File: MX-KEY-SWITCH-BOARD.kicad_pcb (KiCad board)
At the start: 2 copper layers, 97 x 101.2 mm, 112 parts, among them J1 Conn_01x06, J10 Conn_01x06, J11 Conn_01x06, J12 Conn_01x06, J13 Conn_01x06, J14 Conn_01x06, J15 Conn_01x06, J16 Conn_01x06, J17 Conn_01x06, J18 Conn_01x06, J19 Conn_01x06, J2 Conn_01x06, J20 Conn_01x06, J21 Conn_01x06, J22 Conn_01x06, J23 Conn_01x06, J24 Conn_01x06, J25 Conn_01x06, J26 Conn_01x06, J27 Conn_01x06, J28 Conn_01x06, J29 Conn_01x06, J3 Conn_01x06, J30 Conn_01x06, J31 Conn_01x06, J32 Conn_01x06, J33 Conn_01x06, J34 Conn_01x06, J35 Conn_01x06, J36 Conn_01x06, J37 Conn_01x06, J38 Conn_01x06, J39 Conn_01x06, J4 Conn_01x06, J40 Conn_01x06, J41 Conn_01x06, J42 Conn_01x06, J43 Conn_01x06, J44 Conn_01x06, J45 Conn_01x06, J46 Conn_01x06, J47 Conn_01x06, J48 Conn_01x06, J49 Conn_01x06, J5 Conn_01x06, J50 Conn_01x06, J51 Conn_01x06, J52 Conn_01x06, J53 Conn_01x06, J54 Conn_01x06, J55 Conn_01x06, J56 Conn_01x06, J57 Conn_01x06, J58 Conn_01x06, J59 Conn_01x06, J6 Conn_01x06, J60 Conn_01x06, J61 Conn_01x06, J62 Conn_01x06, J63 Conn_01x06, J64 Conn_01x06, J7 Conn_01x06, J8 Conn_01x06, J9 Conn_01x06, SW1 SW_Push, SW10 SW_Push, SW11 SW_Push, SW12 SW_Push, SW13 SW_Push, SW14 SW_Push, SW15 SW_Push, SW16 SW_Push, SW2 SW_Push, SW3 SW_Push, SW4 SW_Push, SW5 SW_Push, SW6 SW_Push, SW7 SW_Push, SW8 SW_Push, SW9 SW_Push

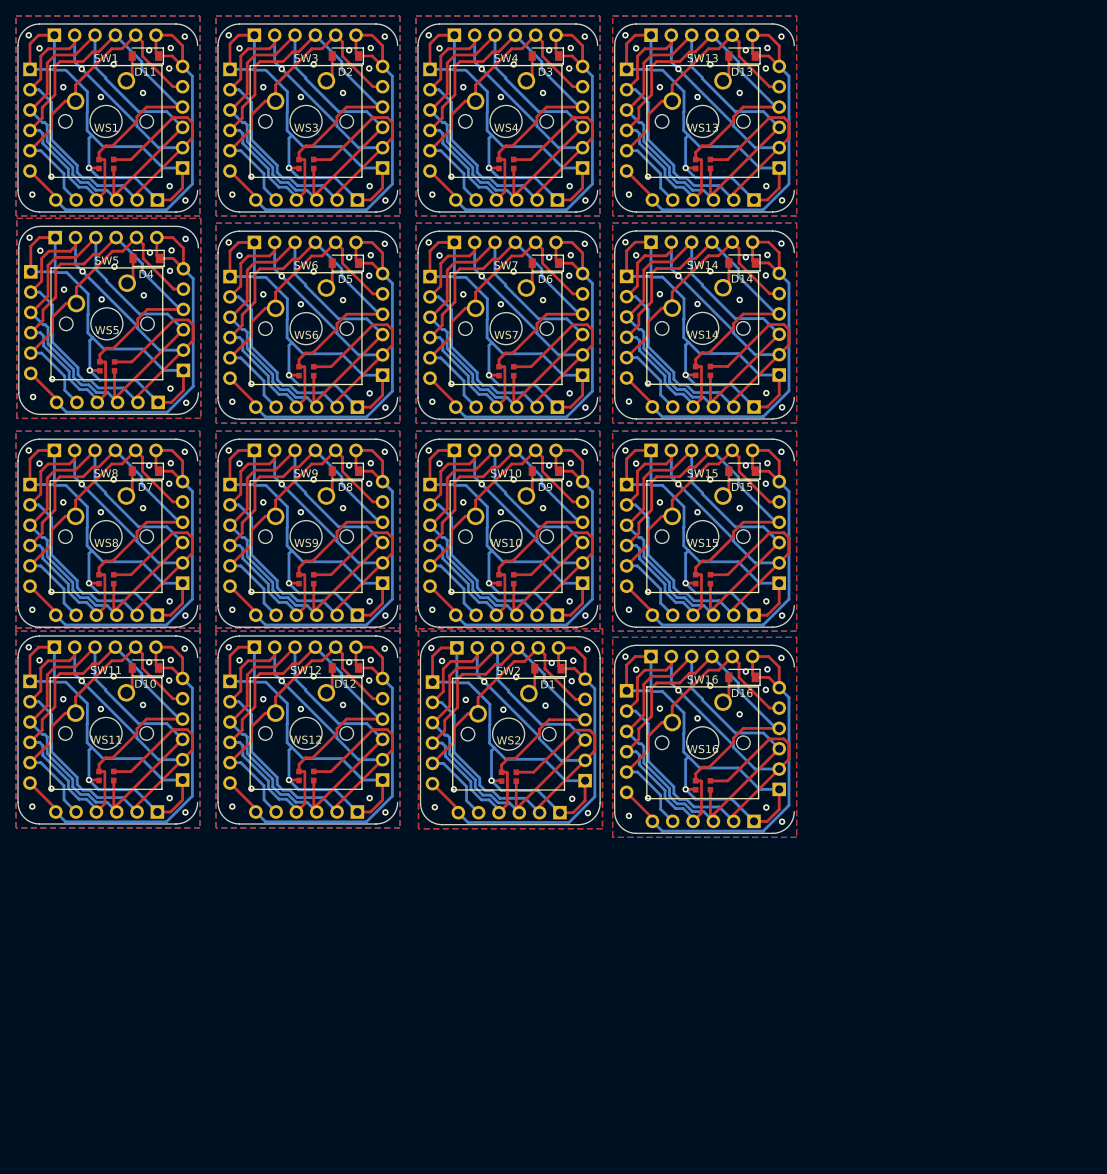
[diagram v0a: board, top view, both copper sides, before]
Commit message: fix
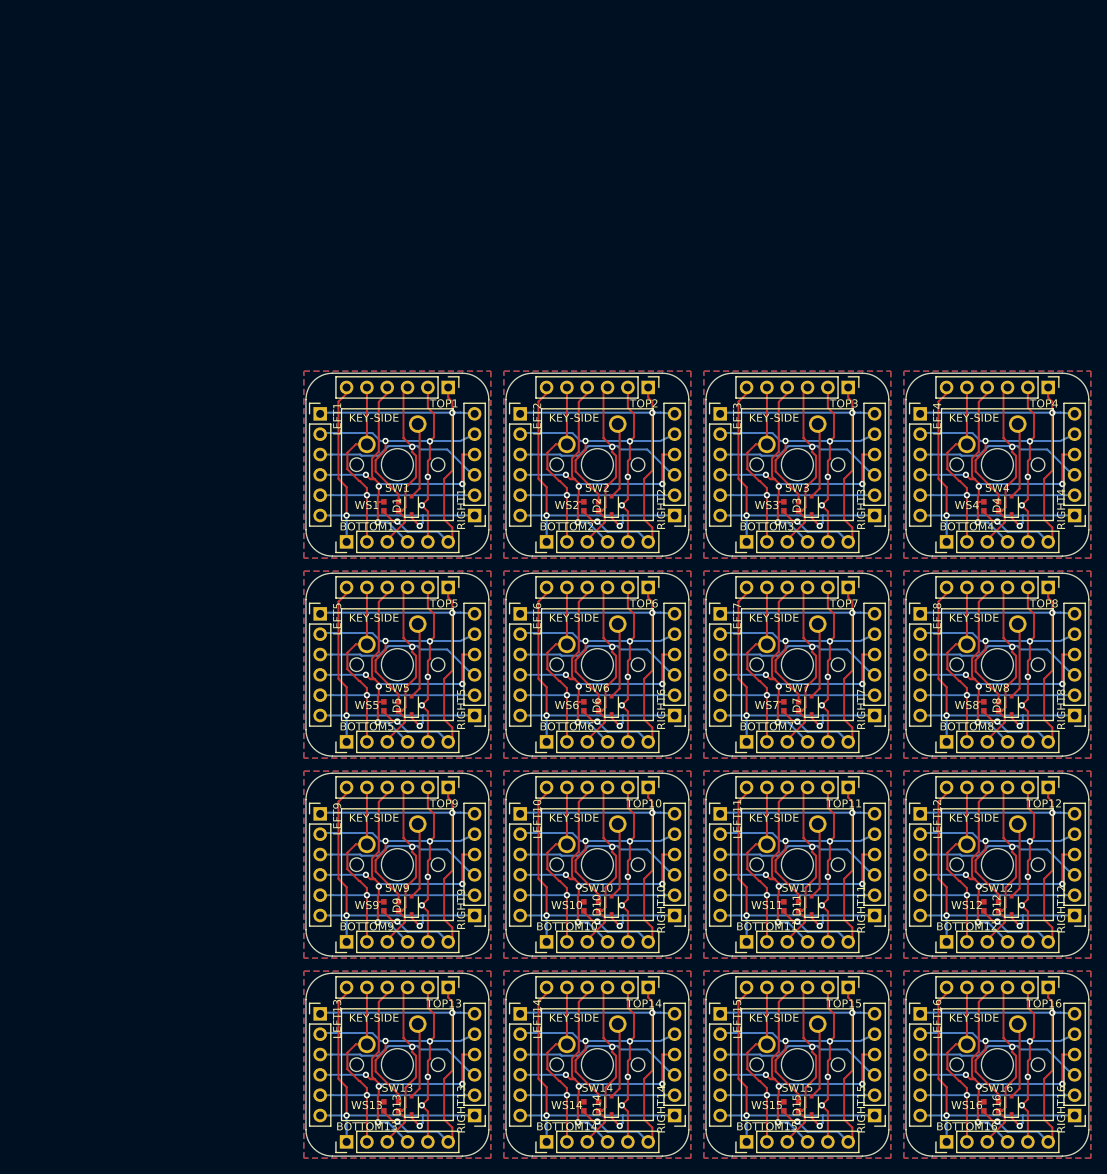
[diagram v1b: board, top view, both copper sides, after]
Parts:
- removed J1, J10, J11, J12, J13, J14, J15, J16, J17, J18, J19, J2, J20, J21, J22, J23, J24, J25, J26, J27, J28, J29, J3, J30, J31, J32, J33, J34, J35, J36, J37, J38, J39, J4, J40, J41, J42, J43, J44, J45, J46, J47, J48, J49, J5, J50, J51, J52, J53, J54, J55, J56, J57, J58, J59, J6, J60, J61, J62, J63, J64, J7, J8, J9: Conn_01x06, Connector_PinHeader_2.54mm:PinHeader_1x06_P2.54mm_Vertical
- added BOTTOM1: Conn_01x06, Connector_PinHeader_2.54mm:PinHeader_1x06_P2.54mm_Vertical, F.Cu at (-8.89, 14.7)
- added BOTTOM10: Conn_01x06, Connector_PinHeader_2.54mm:PinHeader_1x06_P2.54mm_Vertical, F.Cu at (16.1, 64.7)
- added BOTTOM11: Conn_01x06, Connector_PinHeader_2.54mm:PinHeader_1x06_P2.54mm_Vertical, F.Cu at (41.1, 64.7)
- added BOTTOM12: Conn_01x06, Connector_PinHeader_2.54mm:PinHeader_1x06_P2.54mm_Vertical, F.Cu at (66.1, 64.7)
- added BOTTOM13: Conn_01x06, Connector_PinHeader_2.54mm:PinHeader_1x06_P2.54mm_Vertical, F.Cu at (-8.89, 89.7)
- added BOTTOM14: Conn_01x06, Connector_PinHeader_2.54mm:PinHeader_1x06_P2.54mm_Vertical, F.Cu at (16.1, 89.7)
- added BOTTOM15: Conn_01x06, Connector_PinHeader_2.54mm:PinHeader_1x06_P2.54mm_Vertical, F.Cu at (41.1, 89.7)
- added BOTTOM16: Conn_01x06, Connector_PinHeader_2.54mm:PinHeader_1x06_P2.54mm_Vertical, F.Cu at (66.1, 89.7)
- added BOTTOM2: Conn_01x06, Connector_PinHeader_2.54mm:PinHeader_1x06_P2.54mm_Vertical, F.Cu at (16.1, 14.7)
- added BOTTOM3: Conn_01x06, Connector_PinHeader_2.54mm:PinHeader_1x06_P2.54mm_Vertical, F.Cu at (41.1, 14.7)
- added BOTTOM4: Conn_01x06, Connector_PinHeader_2.54mm:PinHeader_1x06_P2.54mm_Vertical, F.Cu at (66.1, 14.7)
- added BOTTOM5: Conn_01x06, Connector_PinHeader_2.54mm:PinHeader_1x06_P2.54mm_Vertical, F.Cu at (-8.89, 39.7)
- added BOTTOM6: Conn_01x06, Connector_PinHeader_2.54mm:PinHeader_1x06_P2.54mm_Vertical, F.Cu at (16.1, 39.7)
- added BOTTOM7: Conn_01x06, Connector_PinHeader_2.54mm:PinHeader_1x06_P2.54mm_Vertical, F.Cu at (41.1, 39.7)
- added BOTTOM8: Conn_01x06, Connector_PinHeader_2.54mm:PinHeader_1x06_P2.54mm_Vertical, F.Cu at (66.1, 39.7)
- added BOTTOM9: Conn_01x06, Connector_PinHeader_2.54mm:PinHeader_1x06_P2.54mm_Vertical, F.Cu at (-8.89, 64.7)
- added LEFT1: Conn_01x06, Connector_PinHeader_2.54mm:PinHeader_1x06_P2.54mm_Vertical, F.Cu at (-12.2, -1.27)
- added LEFT10: Conn_01x06, Connector_PinHeader_2.54mm:PinHeader_1x06_P2.54mm_Vertical, F.Cu at (12.8, 48.7)
- added LEFT11: Conn_01x06, Connector_PinHeader_2.54mm:PinHeader_1x06_P2.54mm_Vertical, F.Cu at (37.8, 48.7)
- added LEFT12: Conn_01x06, Connector_PinHeader_2.54mm:PinHeader_1x06_P2.54mm_Vertical, F.Cu at (62.8, 48.7)
- added LEFT13: Conn_01x06, Connector_PinHeader_2.54mm:PinHeader_1x06_P2.54mm_Vertical, F.Cu at (-12.2, 73.7)
- added LEFT14: Conn_01x06, Connector_PinHeader_2.54mm:PinHeader_1x06_P2.54mm_Vertical, F.Cu at (12.8, 73.7)
- added LEFT15: Conn_01x06, Connector_PinHeader_2.54mm:PinHeader_1x06_P2.54mm_Vertical, F.Cu at (37.8, 73.7)
- added LEFT16: Conn_01x06, Connector_PinHeader_2.54mm:PinHeader_1x06_P2.54mm_Vertical, F.Cu at (62.8, 73.7)
- added LEFT2: Conn_01x06, Connector_PinHeader_2.54mm:PinHeader_1x06_P2.54mm_Vertical, F.Cu at (12.8, -1.27)
- added LEFT3: Conn_01x06, Connector_PinHeader_2.54mm:PinHeader_1x06_P2.54mm_Vertical, F.Cu at (37.8, -1.27)
- added LEFT4: Conn_01x06, Connector_PinHeader_2.54mm:PinHeader_1x06_P2.54mm_Vertical, F.Cu at (62.8, -1.27)
- added LEFT5: Conn_01x06, Connector_PinHeader_2.54mm:PinHeader_1x06_P2.54mm_Vertical, F.Cu at (-12.2, 23.7)
- added LEFT6: Conn_01x06, Connector_PinHeader_2.54mm:PinHeader_1x06_P2.54mm_Vertical, F.Cu at (12.8, 23.7)
- added LEFT7: Conn_01x06, Connector_PinHeader_2.54mm:PinHeader_1x06_P2.54mm_Vertical, F.Cu at (37.8, 23.7)
- added LEFT8: Conn_01x06, Connector_PinHeader_2.54mm:PinHeader_1x06_P2.54mm_Vertical, F.Cu at (62.8, 23.7)
- added LEFT9: Conn_01x06, Connector_PinHeader_2.54mm:PinHeader_1x06_P2.54mm_Vertical, F.Cu at (-12.2, 48.7)
- added RIGHT1: Conn_01x06, Connector_PinHeader_2.54mm:PinHeader_1x06_P2.54mm_Vertical, F.Cu at (7.11, 11.4)
- added RIGHT10: Conn_01x06, Connector_PinHeader_2.54mm:PinHeader_1x06_P2.54mm_Vertical, F.Cu at (32.1, 61.4)
- added RIGHT11: Conn_01x06, Connector_PinHeader_2.54mm:PinHeader_1x06_P2.54mm_Vertical, F.Cu at (57.1, 61.4)
- added RIGHT12: Conn_01x06, Connector_PinHeader_2.54mm:PinHeader_1x06_P2.54mm_Vertical, F.Cu at (82.1, 61.4)
- added RIGHT13: Conn_01x06, Connector_PinHeader_2.54mm:PinHeader_1x06_P2.54mm_Vertical, F.Cu at (7.11, 86.4)
- added RIGHT14: Conn_01x06, Connector_PinHeader_2.54mm:PinHeader_1x06_P2.54mm_Vertical, F.Cu at (32.1, 86.4)
- added RIGHT15: Conn_01x06, Connector_PinHeader_2.54mm:PinHeader_1x06_P2.54mm_Vertical, F.Cu at (57.1, 86.4)
- added RIGHT16: Conn_01x06, Connector_PinHeader_2.54mm:PinHeader_1x06_P2.54mm_Vertical, F.Cu at (82.1, 86.4)
- added RIGHT2: Conn_01x06, Connector_PinHeader_2.54mm:PinHeader_1x06_P2.54mm_Vertical, F.Cu at (32.1, 11.4)
- added RIGHT3: Conn_01x06, Connector_PinHeader_2.54mm:PinHeader_1x06_P2.54mm_Vertical, F.Cu at (57.1, 11.4)
- added RIGHT4: Conn_01x06, Connector_PinHeader_2.54mm:PinHeader_1x06_P2.54mm_Vertical, F.Cu at (82.1, 11.4)
- added RIGHT5: Conn_01x06, Connector_PinHeader_2.54mm:PinHeader_1x06_P2.54mm_Vertical, F.Cu at (7.11, 36.4)
- added RIGHT6: Conn_01x06, Connector_PinHeader_2.54mm:PinHeader_1x06_P2.54mm_Vertical, F.Cu at (32.1, 36.4)
- added RIGHT7: Conn_01x06, Connector_PinHeader_2.54mm:PinHeader_1x06_P2.54mm_Vertical, F.Cu at (57.1, 36.4)
- added RIGHT8: Conn_01x06, Connector_PinHeader_2.54mm:PinHeader_1x06_P2.54mm_Vertical, F.Cu at (82.1, 36.4)
- added RIGHT9: Conn_01x06, Connector_PinHeader_2.54mm:PinHeader_1x06_P2.54mm_Vertical, F.Cu at (7.11, 61.4)
- added TOP1: Conn_01x06, Connector_PinHeader_2.54mm:PinHeader_1x06_P2.54mm_Vertical, F.Cu at (3.81, -4.57)
- added TOP10: Conn_01x06, Connector_PinHeader_2.54mm:PinHeader_1x06_P2.54mm_Vertical, F.Cu at (28.8, 45.4)
- added TOP11: Conn_01x06, Connector_PinHeader_2.54mm:PinHeader_1x06_P2.54mm_Vertical, F.Cu at (53.8, 45.4)
- added TOP12: Conn_01x06, Connector_PinHeader_2.54mm:PinHeader_1x06_P2.54mm_Vertical, F.Cu at (78.8, 45.4)
- added TOP13: Conn_01x06, Connector_PinHeader_2.54mm:PinHeader_1x06_P2.54mm_Vertical, F.Cu at (3.81, 70.4)
- added TOP14: Conn_01x06, Connector_PinHeader_2.54mm:PinHeader_1x06_P2.54mm_Vertical, F.Cu at (28.8, 70.4)
- added TOP15: Conn_01x06, Connector_PinHeader_2.54mm:PinHeader_1x06_P2.54mm_Vertical, F.Cu at (53.8, 70.4)
- added TOP16: Conn_01x06, Connector_PinHeader_2.54mm:PinHeader_1x06_P2.54mm_Vertical, F.Cu at (78.8, 70.4)
- added TOP2: Conn_01x06, Connector_PinHeader_2.54mm:PinHeader_1x06_P2.54mm_Vertical, F.Cu at (28.8, -4.57)
- added TOP3: Conn_01x06, Connector_PinHeader_2.54mm:PinHeader_1x06_P2.54mm_Vertical, F.Cu at (53.8, -4.57)
- added TOP4: Conn_01x06, Connector_PinHeader_2.54mm:PinHeader_1x06_P2.54mm_Vertical, F.Cu at (78.8, -4.57)
- added TOP5: Conn_01x06, Connector_PinHeader_2.54mm:PinHeader_1x06_P2.54mm_Vertical, F.Cu at (3.81, 20.4)
- added TOP6: Conn_01x06, Connector_PinHeader_2.54mm:PinHeader_1x06_P2.54mm_Vertical, F.Cu at (28.8, 20.4)
- added TOP7: Conn_01x06, Connector_PinHeader_2.54mm:PinHeader_1x06_P2.54mm_Vertical, F.Cu at (53.8, 20.4)
- added TOP8: Conn_01x06, Connector_PinHeader_2.54mm:PinHeader_1x06_P2.54mm_Vertical, F.Cu at (78.8, 20.4)
- added TOP9: Conn_01x06, Connector_PinHeader_2.54mm:PinHeader_1x06_P2.54mm_Vertical, F.Cu at (3.81, 45.4)
- D1, D10, D11, D12, D13, D14, D15, D16, D2, D3, D4, D5, D6, D7, D8, D9: value 1N4148W -> Diode-SOD323F; footprint Diode_SMD:D_SOD-123 -> Diode_SMD:D_SOD-323F
- moved D13 137.5 mm to (-0.76, 85.2), turned to 90 degrees
- moved D11 134.9 mm to (49.2, 60.2), turned to 90 degrees
- moved WS13 124.1 mm to (-3.30, 85.3)
- moved SW13 123.9 mm to (0.00, 75.0)
- moved SW8 112.6 mm to (75.0, 25.0)
- moved D4 112.5 mm to (74.2, 10.2), turned to 90 degrees
- moved WS8 111.7 mm to (71.7, 35.3)
- moved D14 106.5 mm to (24.2, 85.2), turned to 90 degrees
- moved WS14 93.0 mm to (21.7, 85.3)
- moved SW14 93.0 mm to (25.0, 75.0)
- moved D12 88.4 mm to (74.2, 60.2), turned to 90 degrees
- moved D7 88.3 mm to (49.2, 35.2), turned to 90 degrees
- moved D8 88.3 mm to (74.2, 35.2), turned to 90 degrees
- moved SW11 88.0 mm to (50.0, 50.0)
- moved SW12 88.0 mm to (75.0, 50.0)
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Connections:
- SW1 pad 1: Net-(D11-Pad2) -> Net-(D1-Pad2)
- SW10 pad 1: Net-(D9-Pad2) -> Net-(D10-Pad2)
- SW11 pad 1: Net-(D10-Pad2) -> Net-(D11-Pad2)
- SW2 pad 1: Net-(D1-Pad2) -> Net-(D2-Pad2)
- SW3 pad 1: Net-(D2-Pad2) -> Net-(D3-Pad2)
- SW4 pad 1: Net-(D3-Pad2) -> Net-(D4-Pad2)
- SW5 pad 1: Net-(D4-Pad2) -> Net-(D5-Pad2)
- SW6 pad 1: Net-(D5-Pad2) -> Net-(D6-Pad2)
- SW7 pad 1: Net-(D6-Pad2) -> Net-(D7-Pad2)
- SW8 pad 1: Net-(D7-Pad2) -> Net-(D8-Pad2)
- SW9 pad 1: Net-(D8-Pad2) -> Net-(D9-Pad2)
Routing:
- net GND: track 1268.1 -> 803.5 mm, vias 240 -> 64
- net DO: track 1059.9 -> 698.5 mm, vias 0 -> 16
- net DI: track 1036.2 -> 730.7 mm, vias 0 -> 64
- net VCC: track 962.4 -> 795.2 mm, vias 16 -> 32
- net ROW: track 828.9 -> 672.8 mm, vias 0 -> 32
- net COL: track 645.4 -> 664.1 mm, vias 0 -> 16
- net Net-(D4-Pad2): track 3.40 -> 9.57 mm
- net Net-(D12-Pad2): track 3.40 -> 9.57 mm
- net Net-(D10-Pad2): track 3.40 -> 9.57 mm
- net Net-(D8-Pad2): track 3.40 -> 9.57 mm
- net Net-(D7-Pad2): track 3.40 -> 9.57 mm
- net Net-(D6-Pad2): track 3.40 -> 9.57 mm
- net Net-(D15-Pad2): track 3.40 -> 9.57 mm
- net Net-(D9-Pad2): track 3.40 -> 9.57 mm
- net Net-(D16-Pad2): track 3.40 -> 9.57 mm
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- added copper zone on F.Cu, net VCC
- removed copper zone on F.Cu, net GND
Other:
- board size 97 x 101.2 mm -> 97.9 x 97.9 mm
- board text added: "(C)WINGTECHCORNER.COM"
- board text added: "KEY-SIDE"
- board text added: "MX-COL2ROW WS2812"
